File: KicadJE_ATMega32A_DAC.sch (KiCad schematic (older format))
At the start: 72 parts, among them J201 CV1, J202 CV2, J203 OUT1, J204 OUT2, J205 IN1, J206 IN2, P201 Doepfer_Power_16pin, SW201 SW_SPDT, U201 TL072, U202 MCP4822

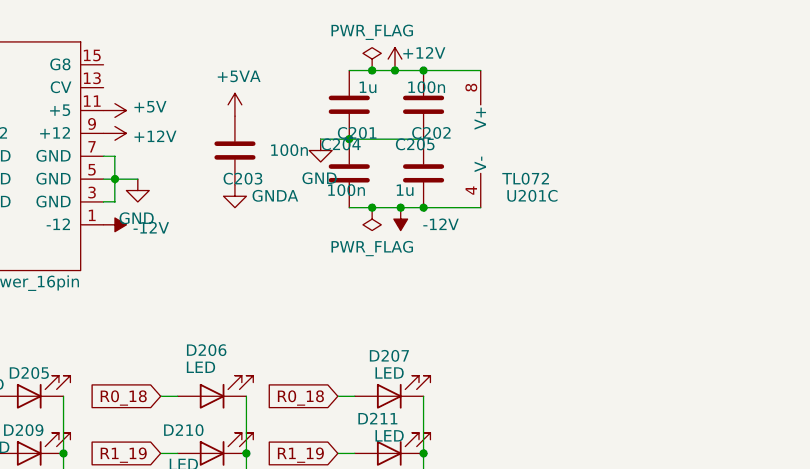
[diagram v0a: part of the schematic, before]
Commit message: 12V PWR
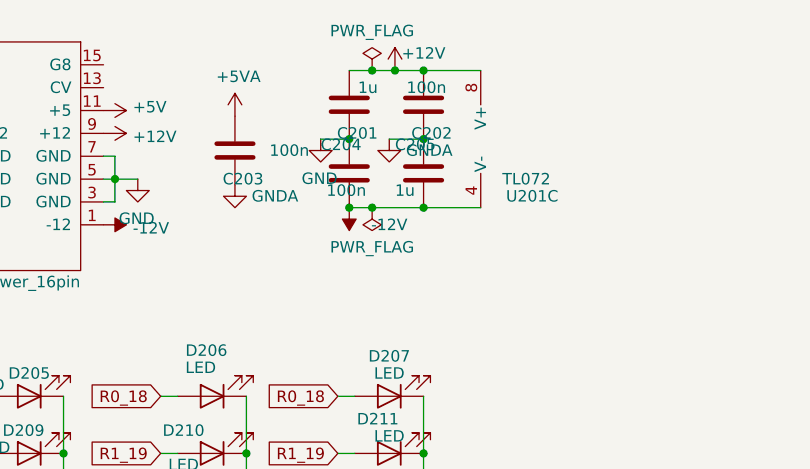
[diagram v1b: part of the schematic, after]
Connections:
- net GND: no longer C202.1, C205.1
- net GNDA: now also C202.1, C205.1
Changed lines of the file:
@@
 L power:-12V #PWR?
 U 1 1 5CE712E5
-P 2750 1250
+P 2525 1250
 AR Path="/5CE712E5" Ref="#PWR?"  Part="1"
 AR Path="/5CD3F059/5CE712E5" Ref="#PWR?"  Part="1"
 AR Path="/5CE3E7A9/5CE712E5" Ref="#PWR0215"  Part="1"
-F 0 "#PWR0215" H 2750 1350 50  0001 C CNN
-F 1 "-12V" H 2575 1325 50  0000 C CNN
-F 2 "" H 2750 1250 50  0001 C CNN
-F 3 "" H 2750 1250 50  0001 C CNN
-	1    2750 1250
+F 0 "#PWR0215" H 2525 1350 50  0001 C CNN
+F 1 "-12V" H 2350 1325 50  0000 C CNN
+F 2 "" H 2525 1250 50  0001 C CNN
+F 3 "" H 2525 1250 50  0001 C CNN
+	1    2525 1250
 	-1   0    0    1
 $EndComp
@@
 Wire Wire Line
 	2400 950  2525 950
-Wire Wire Line
-	2625 1250 2750 1250
 Wire Wire Line
 	1275 2075 1275 2325
@@
 Connection ~ 2525 950
 Wire Wire Line
-	2525 950  2850 950
-Wire Wire Line
 	2525 1250 2625 1250
 Connection ~ 2625 1250
@@
 Wire Wire Line
 	2850 1250 3100 1250
-Connection ~ 2750 1250
-Wire Wire Line
-	2750 1250 2850 1250
 Wire Wire Line
 	2625 650  2725 650
@@
 Wire Wire Line
 	9275 1350 9325 1350
+Connection ~ 2525 1250
+Wire Wire Line
+	2625 1250 2850 1250
+$Comp
+L power:GNDA #PWR?
+U 1 1 5D433FC3
+P 2700 950
+AR Path="/5D433FC3" Ref="#PWR?"  Part="1"
+AR Path="/5CD3F059/5D433FC3" Ref="#PWR?"  Part="1"
+AR Path="/5CE3E7A9/5D433FC3" Ref="#PWR?"  Part="1"
+F 0 "#PWR?" H 2700 700 50  0001 C CNN
+F 1 "GNDA" H 2875 900 50  0000 C CNN
+F 2 "" H 2700 950 50  0001 C CNN
+F 3 "" H 2700 950 50  0001 C CNN
+	1    2700 950
+	1    0    0    -1
+$EndComp
+Wire Wire Line
+	2700 950  2850 950
+Connection ~ 2850 950
 $EndSCHEMATC

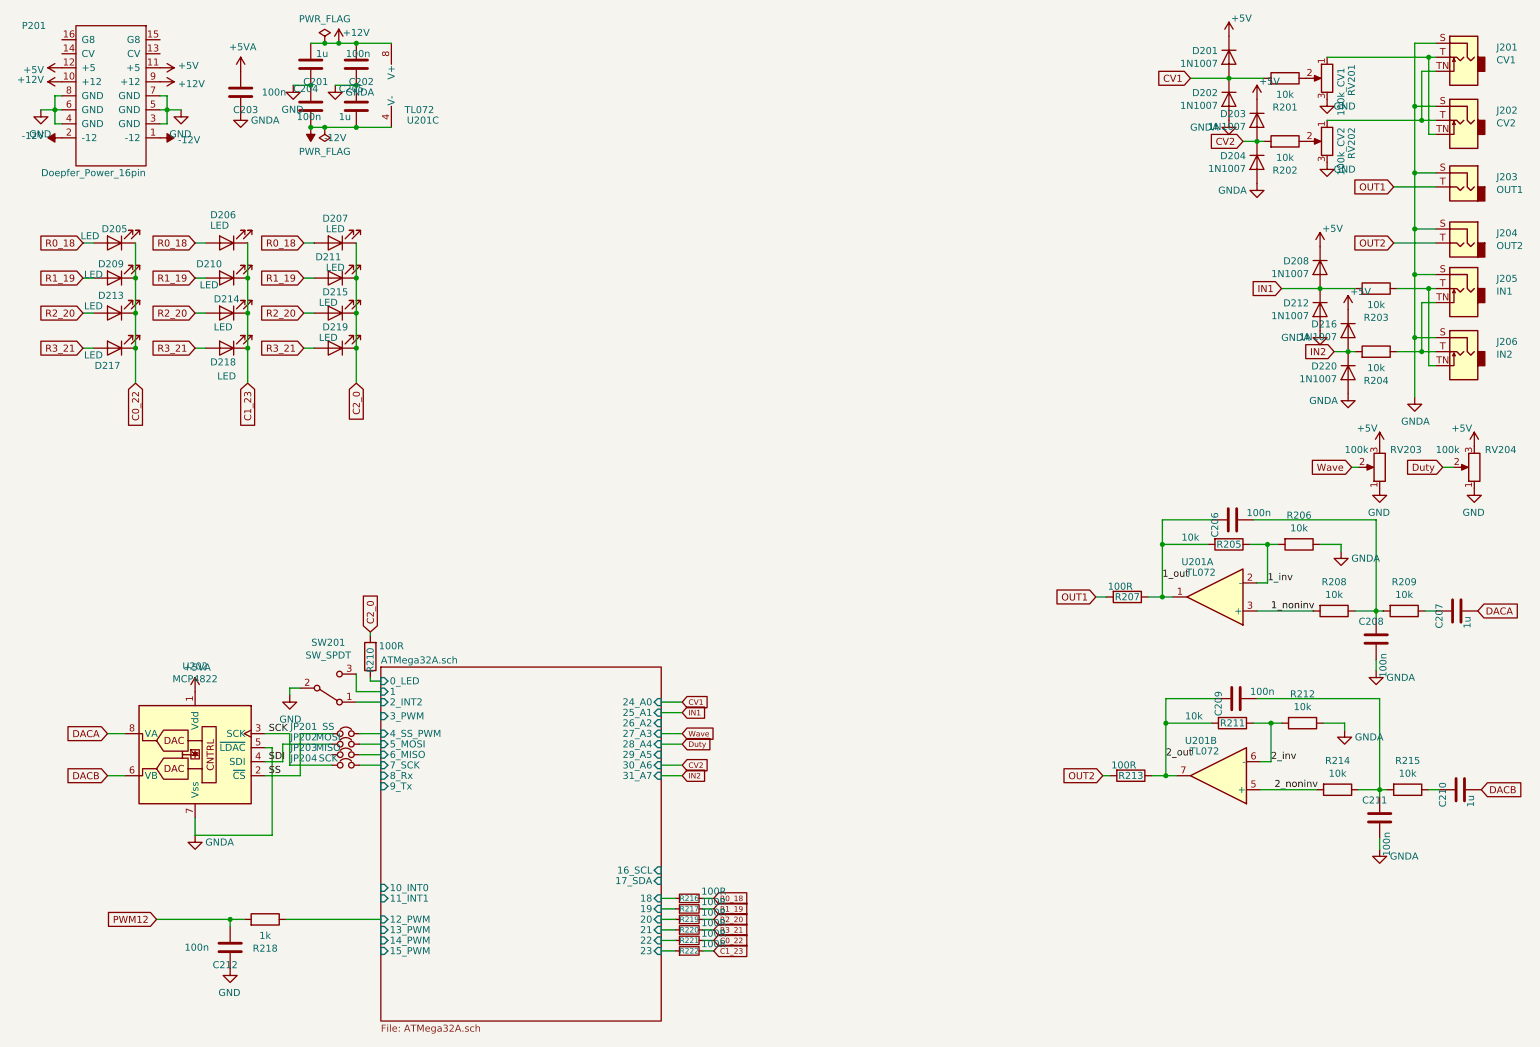
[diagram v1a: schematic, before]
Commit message: Routed
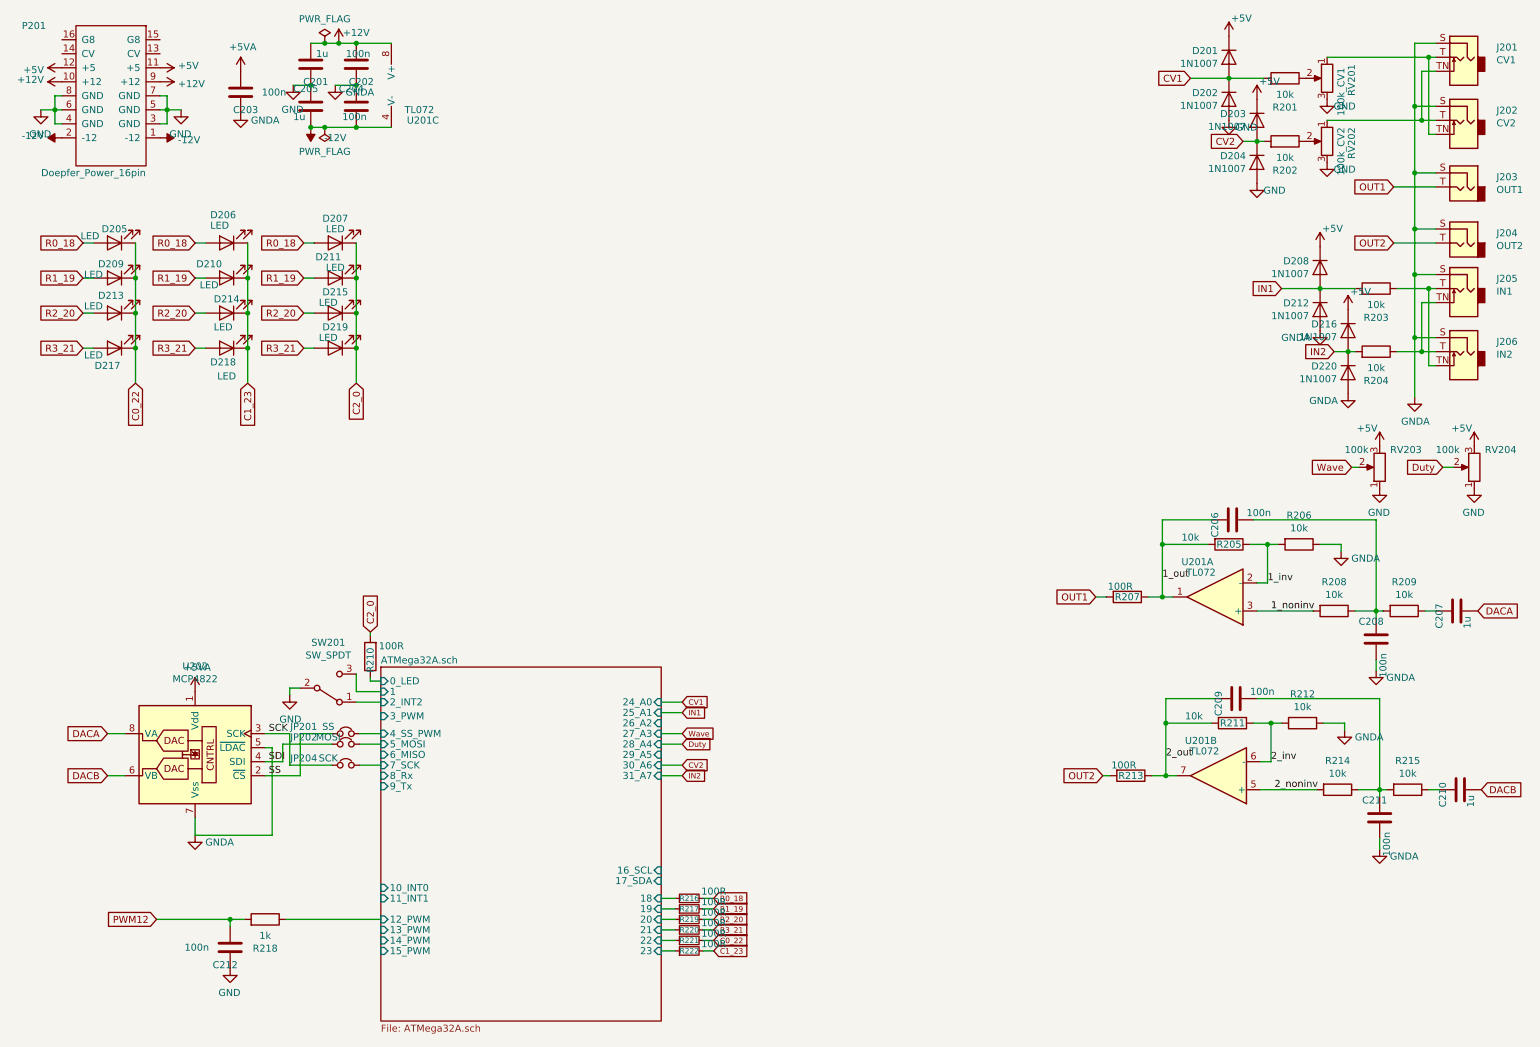
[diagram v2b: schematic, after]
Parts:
- removed JP203: MISO, Connector_PinSocket_2.54mm:PinSocket_1x02_P2.54mm_Vertical, symbol Device:Jumper_NC_Small
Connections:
- net GND: now also C205.1, D202.2 (A), D204.2 (A); no longer C204.1
- net GNDA: now also C204.1; no longer C205.1, D202.2 (A), D204.2 (A)
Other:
- moved on the sheet: C204, C205
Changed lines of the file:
@@
 	10400 2300 10400 2750
-$Comp
-L power:GNDA #PWR?
-U 1 1 5CDD4247
-P 9075 1200
-AR Path="/5CDD4247" Ref="#PWR?"  Part="1"
-AR Path="/5CD3F059/5CDD4247" Ref="#PWR?"  Part="1"
-AR Path="/5CE3E7A9/5CDD4247" Ref="#PWR0214"  Part="1"
-F 0 "#PWR0214" H 9075 950 50  0001 C CNN
-F 1 "GNDA" H 9250 1150 50  0000 C CNN
-F 2 "" H 9075 1200 50  0001 C CNN
-F 3 "" H 9075 1200 50  0001 C CNN
-	1    9075 1200
-	-1   0    0    -1
-$EndComp
 $Comp
 L Analog_DAC:MCP4822 U202
@@
 L Device:C C?
 U 1 1 5CE712D0
-P 2525 1100
+P 2850 1100
 AR Path="/5CE712D0" Ref="C?"  Part="1"
 AR Path="/5CD3F059/5CE712D0" Ref="C?"  Part="1"
 AR Path="/5CE3E7A9/5CE712D0" Ref="C204"  Part="1"
-F 0 "C204" H 2400 1225 50  0000 L CNN
-F 1 "100n" H 2425 1025 50  0000 L CNN
-F 2 "Capacitor_SMD:C_0805_2012Metric_Pad1.15x1.40mm_HandSolder" H 2563 950 50  0001 C CNN
-F 3 "~" H 2525 1100 50  0001 C CNN
-	1    2525 1100
+F 0 "C204" H 2725 1225 50  0000 L CNN
+F 1 "100n" H 2750 1025 50  0000 L CNN
+F 2 "Capacitor_SMD:C_0805_2012Metric_Pad1.15x1.40mm_HandSolder" H 2888 950 50  0001 C CNN
+F 3 "~" H 2850 1100 50  0001 C CNN
+	1    2850 1100
 	1    0    0    -1
 $EndComp
@@
 L Device:C C?
 U 1 1 5CE712D6
-P 2850 1100
+P 2525 1100
 AR Path="/5CE712D6" Ref="C?"  Part="1"
 AR Path="/5CD3F059/5CE712D6" Ref="C?"  Part="1"
 AR Path="/5CE3E7A9/5CE712D6" Ref="C205"  Part="1"
-F 0 "C205" H 2725 1225 50  0000 L CNN
-F 1 "1u" H 2725 1025 50  0000 L CNN
-F 2 "Capacitor_SMD:C_1206_3216Metric_Pad1.42x1.75mm_HandSolder" H 2888 950 50  0001 C CNN
-F 3 "~" H 2850 1100 50  0001 C CNN
-	1    2850 1100
+F 0 "C205" H 2400 1225 50  0000 L CNN
+F 1 "1u" H 2400 1025 50  0000 L CNN
+F 2 "Capacitor_SMD:C_1206_3216Metric_Pad1.42x1.75mm_HandSolder" H 2563 950 50  0001 C CNN
+F 3 "~" H 2525 1100 50  0001 C CNN
+	1    2525 1100
 	1    0    0    -1
 $EndComp
@@
 	1    9475 1350
 	0    1    -1   0
-$EndComp
-$Comp
-L power:GNDA #PWR?
-U 1 1 5D605339
-P 9275 1650
-AR Path="/5D605339" Ref="#PWR?"  Part="1"
-AR Path="/5CD3F059/5D605339" Ref="#PWR?"  Part="1"
-AR Path="/5CE3E7A9/5D605339" Ref="#PWR0219"  Part="1"
-F 0 "#PWR0219" H 9275 1400 50  0001 C CNN
-F 1 "GNDA" H 9450 1600 50  0000 C CNN
-F 2 "" H 9275 1650 50  0001 C CNN
-F 3 "" H 9275 1650 50  0001 C CNN
-	1    9275 1650
-	-1   0    0    -1
 $EndComp
 $Comp
@@
 Text Label 2225 5575 0    50   ~ 0
 SCK
-$Comp
-L Device:Jumper_NC_Small JP203
-U 1 1 5D23F56B
-P 2775 5725
-F 0 "JP203" H 2475 5775 50  0000 C CNN
-F 1 "MISO" H 2650 5775 50  0000 C CNN
-F 2 "Connector_PinSocket_2.54mm:PinSocket_1x02_P2.54mm_Vertical" H 2775 5725 50  0001 C CNN
-F 3 "~" H 2775 5725 50  0001 C CNN
-	1    2775 5725
-	1    0    0    -1
-$EndComp
-Wire Wire Line
-	2875 5725 3025 5725
 Text GLabel 1700 2075 0    50   Input ~ 0
 R0_18
@@
 Text GLabel 5400 6975 2    39   Input ~ 0
 R3_21
-Connection ~ 2525 950
 Wire Wire Line
 	2525 1250 2625 1250
 Connection ~ 2625 1250
-Connection ~ 2850 1250
-Wire Wire Line
-	2850 1250 3100 1250
 Wire Wire Line
 	2625 650  2725 650
@@
 Wire Wire Line
 	9275 1350 9325 1350
-Connection ~ 2525 1250
-Wire Wire Line
-	2625 1250 2850 1250
 $Comp
 L power:GNDA #PWR?
@@
 AR Path="/5D433FC3" Ref="#PWR?"  Part="1"
 AR Path="/5CD3F059/5D433FC3" Ref="#PWR?"  Part="1"
-AR Path="/5CE3E7A9/5D433FC3" Ref="#PWR?"  Part="1"
-F 0 "#PWR?" H 2700 700 50  0001 C CNN
+AR Path="/5CE3E7A9/5D433FC3" Ref="#PWR0101"  Part="1"
+F 0 "#PWR0101" H 2700 700 50  0001 C CNN
 F 1 "GNDA" H 2875 900 50  0000 C CNN
 F 2 "" H 2700 950 50  0001 C CNN
@@
 Wire Wire Line
 	2700 950  2850 950
+Wire Wire Line
+	2625 1250 2850 1250
 Connection ~ 2850 950
+Connection ~ 2850 1250
+Wire Wire Line
+	2850 1250 3100 1250
+Connection ~ 2525 950
+Connection ~ 2525 1250
+$Comp
+L Envelope-cache-2018-08-04-13-00-04:GND #PWR?
+U 1 1 5D4C4D4B
+P 9275 1650
+F 0 "#PWR?" H 9275 1400 50  0001 C CNN
+F 1 "GND" H 9150 1600 50  0000 C CNN
+F 2 "" H 9275 1650 50  0001 C CNN
+F 3 "" H 9275 1650 50  0001 C CNN
+	1    9275 1650
+	-1   0    0    -1
+$EndComp
+$Comp
+L Envelope-cache-2018-08-04-13-00-04:GND #PWR?
+U 1 1 5D4C4F62
+P 9075 1200
+F 0 "#PWR?" H 9075 950 50  0001 C CNN
+F 1 "GND" H 8950 1150 50  0000 C CNN
+F 2 "" H 9075 1200 50  0001 C CNN
+F 3 "" H 9075 1200 50  0001 C CNN
+	1    9075 1200
+	-1   0    0    -1
+$EndComp
 $EndSCHEMATC
